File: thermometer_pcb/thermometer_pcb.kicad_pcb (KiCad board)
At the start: 2 copper layers, 76.6 x 49 mm, 23 parts, among them J1 POWER_IN, J2 TC_IN, J3 EXT_DS1, J4 EXT_DS2, J5 DISP, J6 Conn_01x02, J7 SPI, J8 I2C, J9 ENC, Q1 PN2222A, Q2 PN2222A, U1 DS18B20

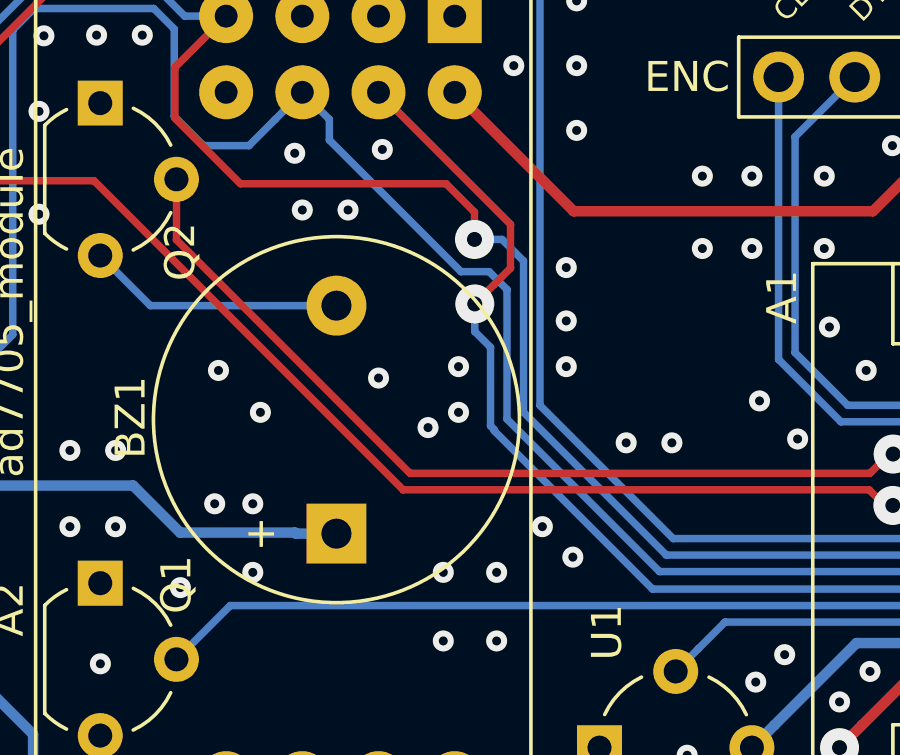
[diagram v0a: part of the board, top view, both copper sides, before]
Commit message: pcb: align some tracks
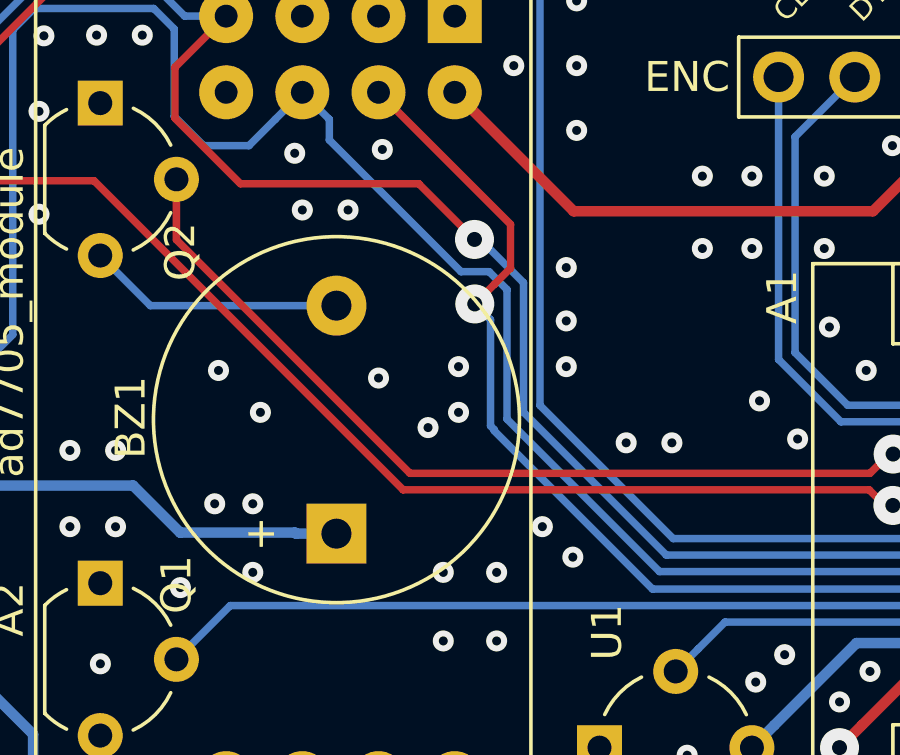
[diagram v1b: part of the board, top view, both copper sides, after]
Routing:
- net /12(MISO): track 98.0 -> 97.1 mm
